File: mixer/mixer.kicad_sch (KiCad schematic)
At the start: 6 parts, among them J10 C_BOARD_IN_1, J11 C_BOARD_IN_2, J12 M_BOARD_IN_1, J13 M_BOARD_IN_2, J14 C_BOARD_OUT_1, J15 C_BOARD_OUT_2

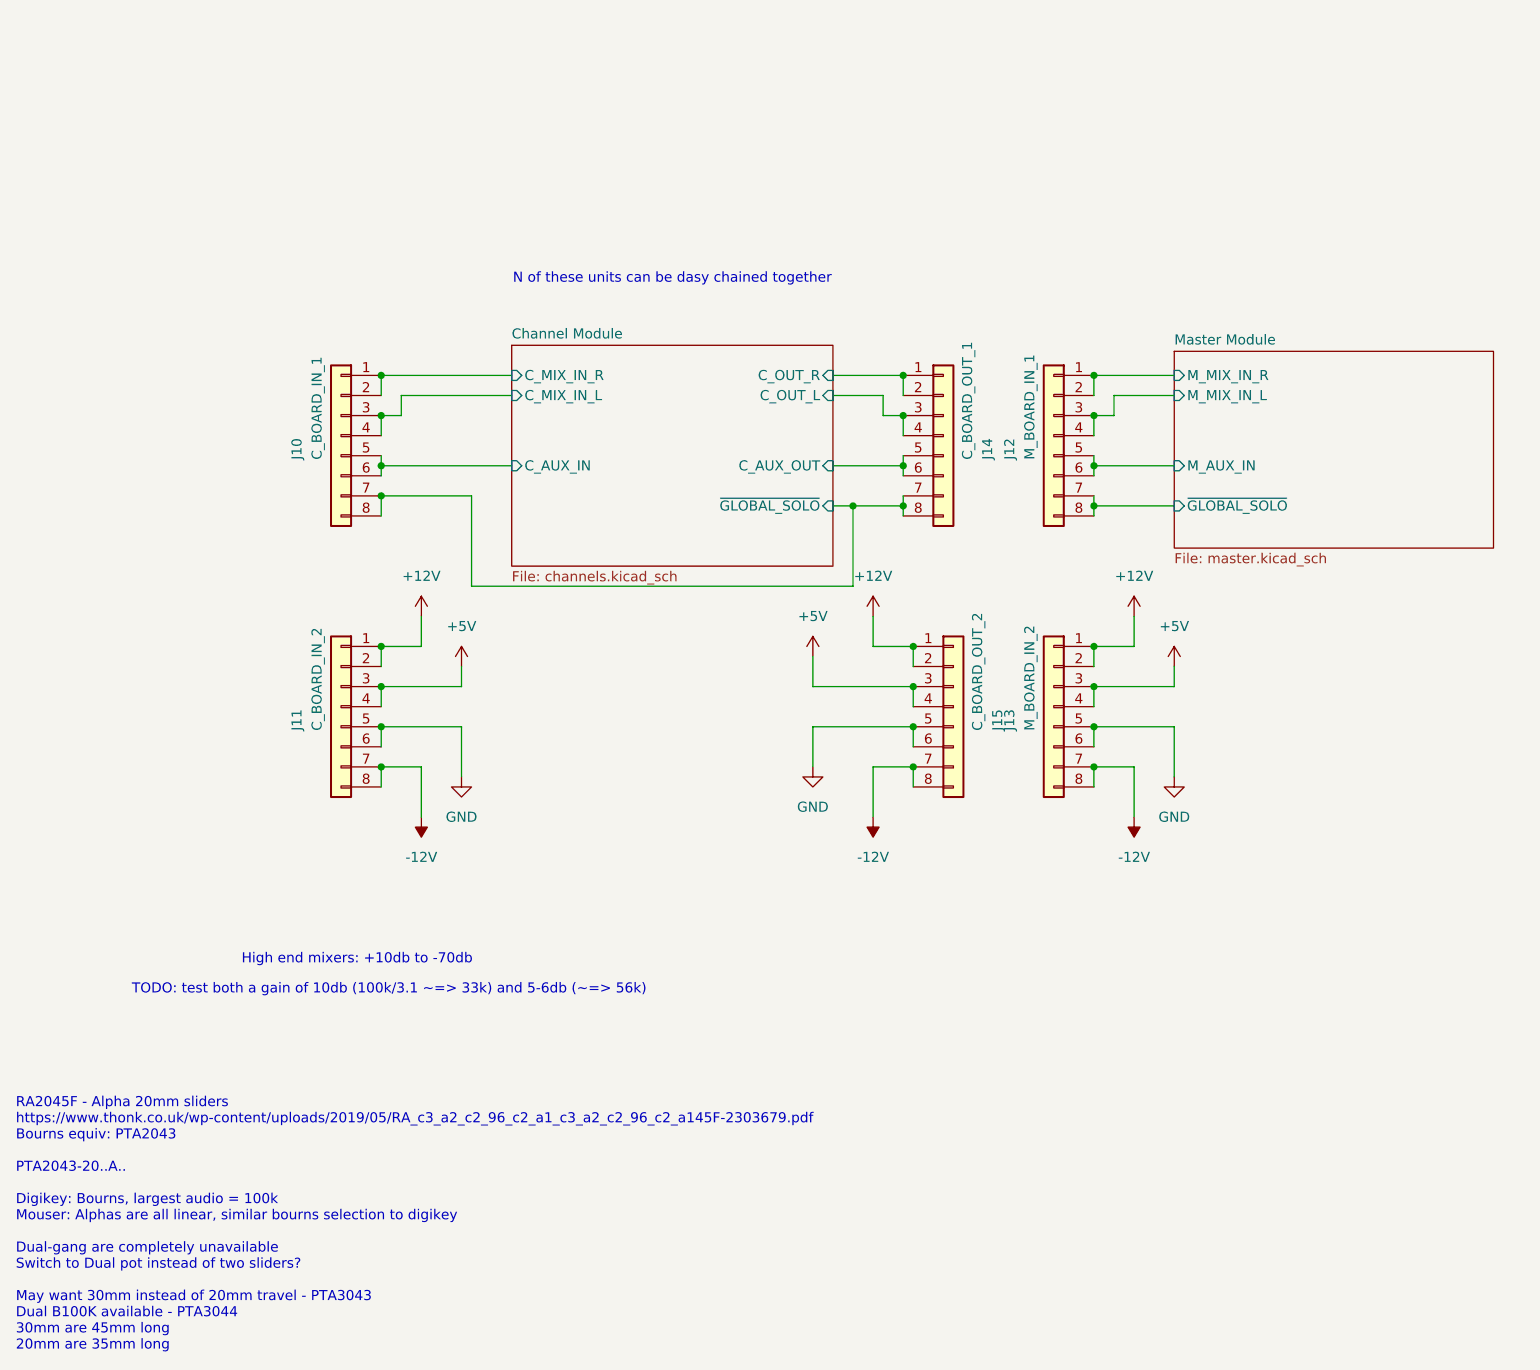
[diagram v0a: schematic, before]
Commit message: layed out parts
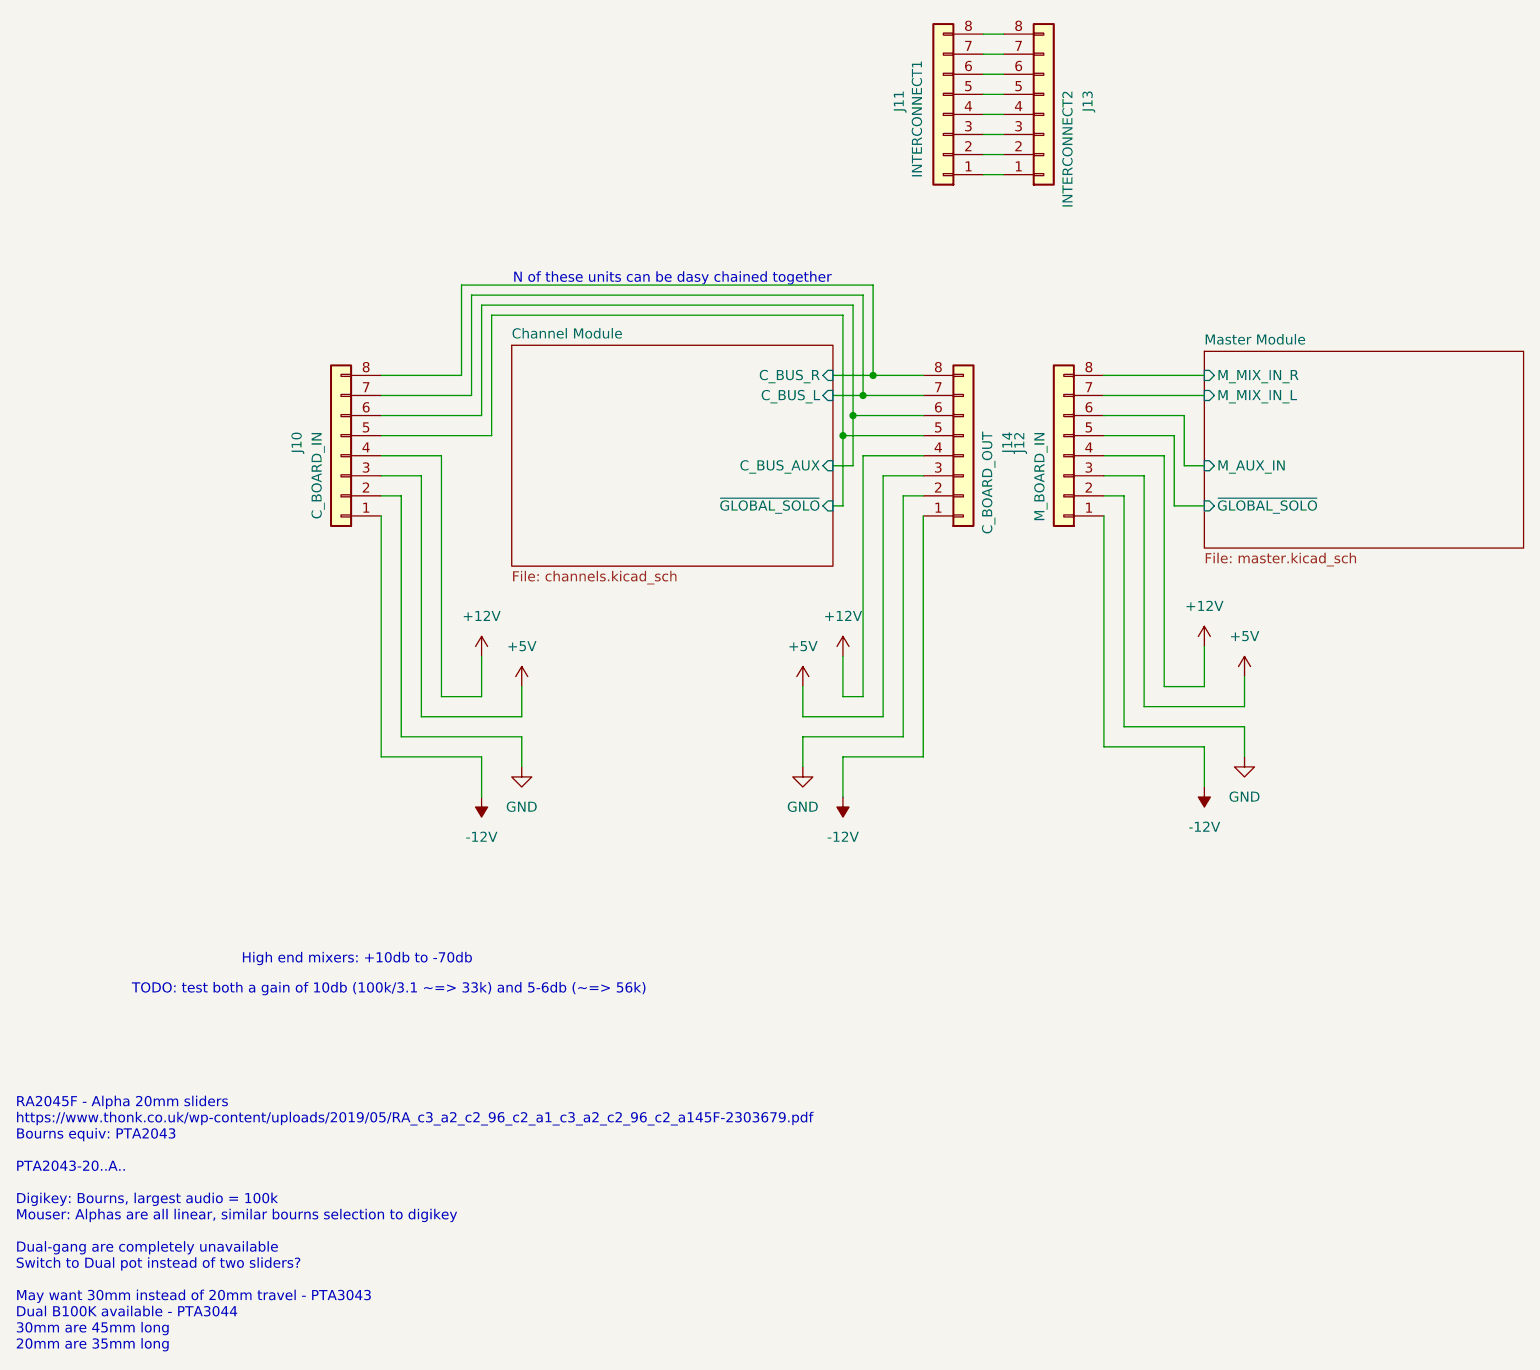
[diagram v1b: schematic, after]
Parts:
- removed J15: C_BOARD_OUT_2, Connector_PinHeader_2.54mm:PinHeader_2x04_P2.54mm_Horizontal, symbol Connector_Generic:Conn_01x08
- J10: value C_BOARD_IN_1 -> C_BOARD_IN; footprint Connector_PinSocket_2.54mm:PinSocket_2x04_P2.54mm_Horizontal -> Connector_PinHeader_1.27mm:PinHeader_1x08_P1.27mm_Vertical
- J11: value C_BOARD_IN_2 -> INTERCONNECT1; footprint Connector_PinSocket_2.54mm:PinSocket_2x04_P2.54mm_Horizontal -> Connector_PinHeader_1.27mm:PinHeader_1x08_P1.27mm_Vertical
- J12: value M_BOARD_IN_1 -> M_BOARD_IN; footprint Connector_PinSocket_2.54mm:PinSocket_2x04_P2.54mm_Horizontal -> Connector_PinSocket_1.27mm:PinSocket_1x08_P1.27mm_Vertical
- J13: value M_BOARD_IN_2 -> INTERCONNECT2; footprint Connector_PinSocket_2.54mm:PinSocket_2x04_P2.54mm_Horizontal -> Connector_PinHeader_1.27mm:PinHeader_1x08_P1.27mm_Vertical
- J14: value C_BOARD_OUT_1 -> C_BOARD_OUT; footprint Connector_PinHeader_2.54mm:PinHeader_2x04_P2.54mm_Horizontal -> Connector_PinSocket_1.27mm:PinSocket_1x08_P1.27mm_Vertical
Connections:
- net +12V: now also J10.4 (Pin_4), J12.4 (Pin_4), J14.4 (Pin_4); no longer J11.1 (Pin_1), J11.2 (Pin_2), J13.1 (Pin_1), J13.2 (Pin_2)
- net +5V: now also J10.3 (Pin_3), J12.3 (Pin_3), J14.3 (Pin_3); no longer J11.3 (Pin_3), J11.4 (Pin_4), J13.3 (Pin_3), J13.4 (Pin_4)
- net -12V: now also J10.1 (Pin_1), J12.1 (Pin_1), J14.1 (Pin_1); no longer J11.7 (Pin_7), J11.8 (Pin_8), J13.7 (Pin_7), J13.8 (Pin_8)
- net Channel Module/~{GLOBAL_SOLO}: now also J10.5 (Pin_5), J14.5 (Pin_5); no longer J10.7 (Pin_7), J10.8 (Pin_8), J14.7 (Pin_7), J14.8 (Pin_8)
- net GND: now also J10.2 (Pin_2), J12.2 (Pin_2), J14.2 (Pin_2); no longer J11.5 (Pin_5), J11.6 (Pin_6), J13.5 (Pin_5), J13.6 (Pin_6)
- net Master Module/M_AUX_IN: no longer J12.5 (Pin_5)
- net Master Module/M_MIX_IN_L: now also J12.7 (Pin_7); no longer J12.3 (Pin_3), J12.4 (Pin_4)
- net Master Module/M_MIX_IN_R: now also J12.8 (Pin_8); no longer J12.1 (Pin_1), J12.2 (Pin_2)
- net Master Module/~{GLOBAL_SOLO}: now also J12.5 (Pin_5); no longer J12.7 (Pin_7), J12.8 (Pin_8)
- net Channel Module/C_AUX_IN renamed Channel Module/C_BUS_AUX
- net Channel Module/C_BUS_AUX: now also J14.6 (Pin_6); no longer J10.5 (Pin_5)
- removed net Channel Module/C_AUX_OUT: J14.5 (Pin_5), J14.6 (Pin_6)
- removed net Channel Module/C_MIX_IN_L: J10.3 (Pin_3), J10.4 (Pin_4)
- removed net Channel Module/C_MIX_IN_R: J10.1 (Pin_1), J10.2 (Pin_2)
- removed net Channel Module/C_OUT_L: J14.3 (Pin_3), J14.4 (Pin_4)
- removed net Channel Module/C_OUT_R: J14.1 (Pin_1), J14.2 (Pin_2)
- new net: J11.1 (Pin_1), J13.1 (Pin_1)
- new net: J11.2 (Pin_2), J13.2 (Pin_2)
- new net: J11.3 (Pin_3), J13.3 (Pin_3)
- new net: J11.4 (Pin_4), J13.4 (Pin_4)
- new net: J11.5 (Pin_5), J13.5 (Pin_5)
- new net: J11.6 (Pin_6), J13.6 (Pin_6)
- new net: J11.7 (Pin_7), J13.7 (Pin_7)
- new net: J11.8 (Pin_8), J13.8 (Pin_8)
- new net Channel Module/C_BUS_L: J10.7 (Pin_7), J14.7 (Pin_7)
- new net Channel Module/C_BUS_R: J10.8 (Pin_8), J14.8 (Pin_8)
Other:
- sheet Channel Module ports: added C_BUS_AUX, C_BUS_L, C_BUS_R; removed C_AUX_IN, C_AUX_OUT, C_MIX_IN_L, C_MIX_IN_R, C_OUT_L, C_OUT_R
- moved on the sheet: J10, J12, J14

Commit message: layout master board
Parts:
- J10: footprint Connector_PinHeader_1.27mm:PinHeader_1x08_P1.27mm_Vertical -> Connector_PinSocket_1.27mm:PinSocket_1x08_P1.27mm_Vertical
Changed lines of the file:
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@@
 			)
 		)
-		(property "Footprint" "Connector_PinHeader_1.27mm:PinHeader_1x08_P1.27mm_Vertical"
+		(property "Footprint" "Connector_PinSocket_1.27mm:PinSocket_1x08_P1.27mm_Vertical"
 			(at 72.39 72.39 0)
 			(effects
